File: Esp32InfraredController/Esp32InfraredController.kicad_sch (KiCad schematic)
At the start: 6 parts, among them J1 Conn_02x05_Odd_Even, Q1 SS8050, U1 ESP32-C3_SUPERMINI_SMD

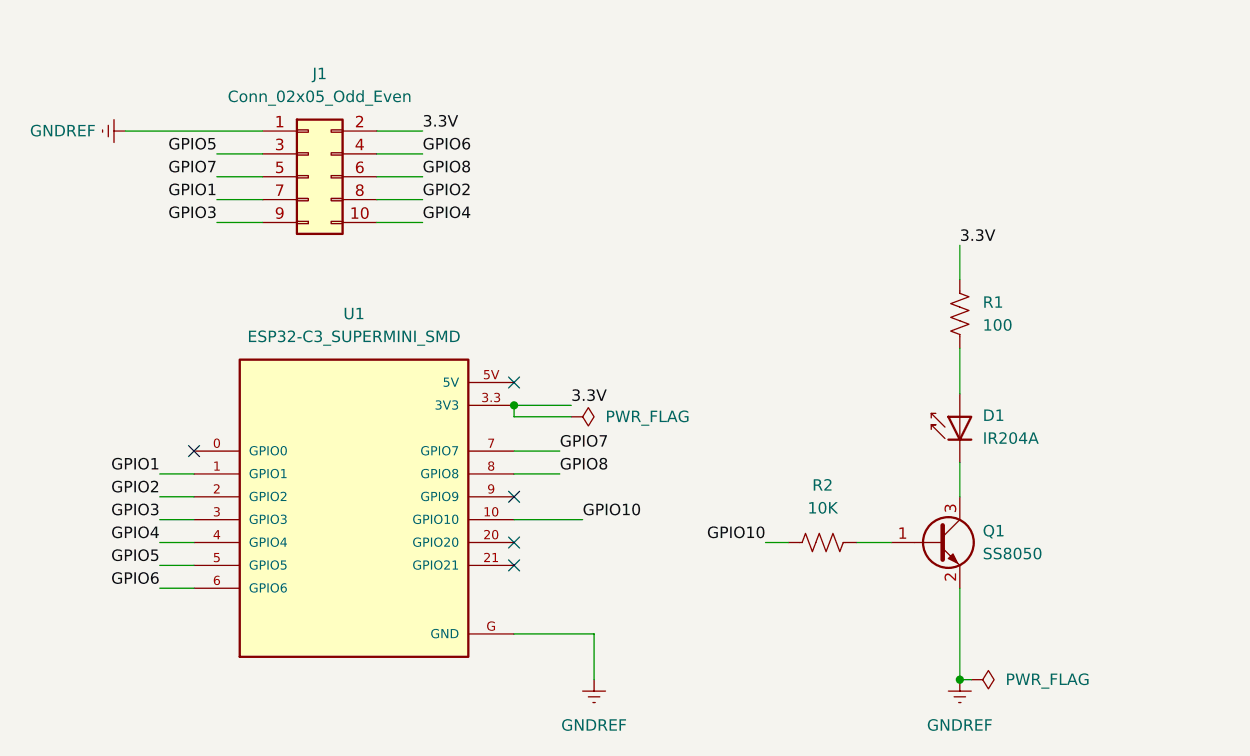
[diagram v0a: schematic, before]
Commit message: no message
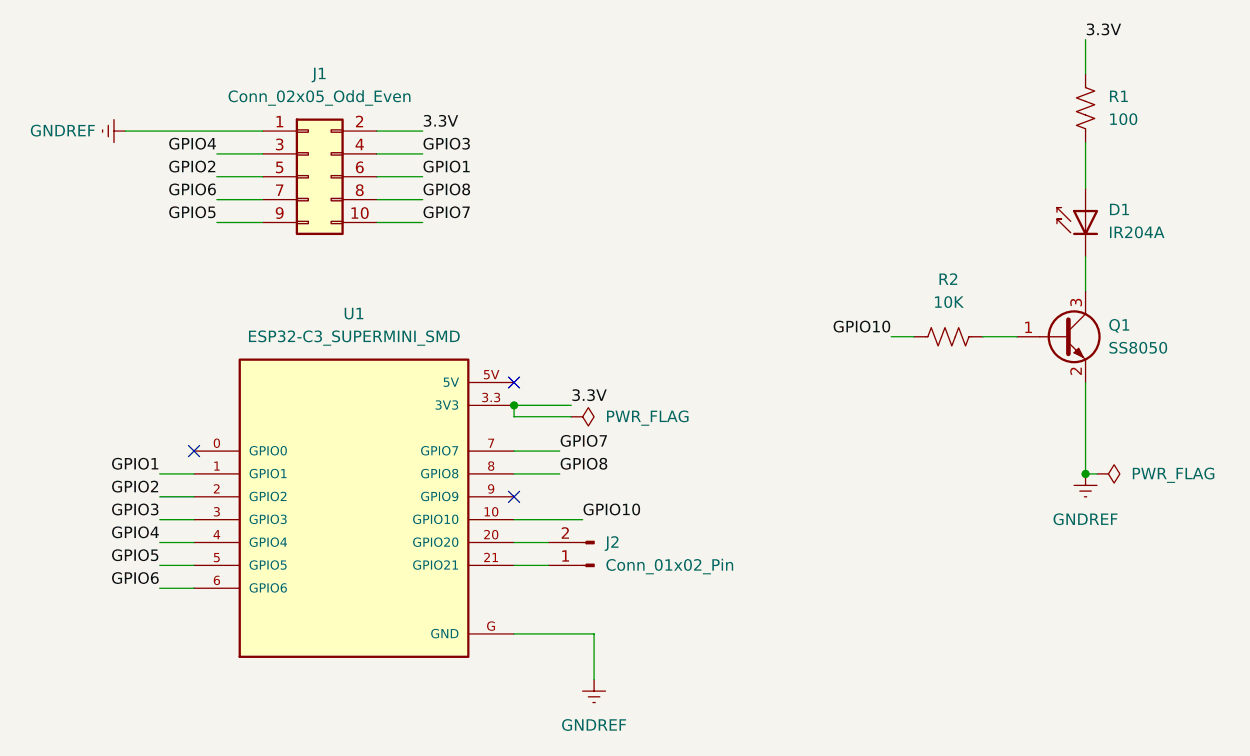
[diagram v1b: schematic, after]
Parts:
- added J2: Conn_01x02_Pin, Connector_PinHeader_1.00mm:PinHeader_1x02_P1.00mm_Vertical, symbol Connector:Conn_01x02_Pin
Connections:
- net GPIO1: now also J1.6 (Pin_6); no longer J1.7 (Pin_7)
- net GPIO2: now also J1.5 (Pin_5); no longer J1.8 (Pin_8)
- net GPIO3: now also J1.4 (Pin_4); no longer J1.9 (Pin_9)
- net GPIO4: now also J1.3 (Pin_3); no longer J1.10 (Pin_10)
- net GPIO5: now also J1.9 (Pin_9); no longer J1.3 (Pin_3)
- net GPIO6: now also J1.7 (Pin_7); no longer J1.4 (Pin_4)
- net GPIO7: now also J1.10 (Pin_10); no longer J1.5 (Pin_5)
- net GPIO8: now also J1.8 (Pin_8); no longer J1.6 (Pin_6)
- net at U1.20 (GPIO20): now also J2.2 (Pin_2)
- net at U1.21 (GPIO21): now also J2.1 (Pin_1)
- no-connect marks 5 -> 3
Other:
- moved on the sheet: D1, Q1, R1, R2
